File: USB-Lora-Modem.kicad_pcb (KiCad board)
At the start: 4 copper layers, 38.5 x 50.5 mm, 29 parts, among them J2 USB_JUMPER, SW1 KILL_SWITCH, U1 E22-900T30S, U4 USBLC6-2SC6, U6 TPS62A01ADRL, U7 CH343P

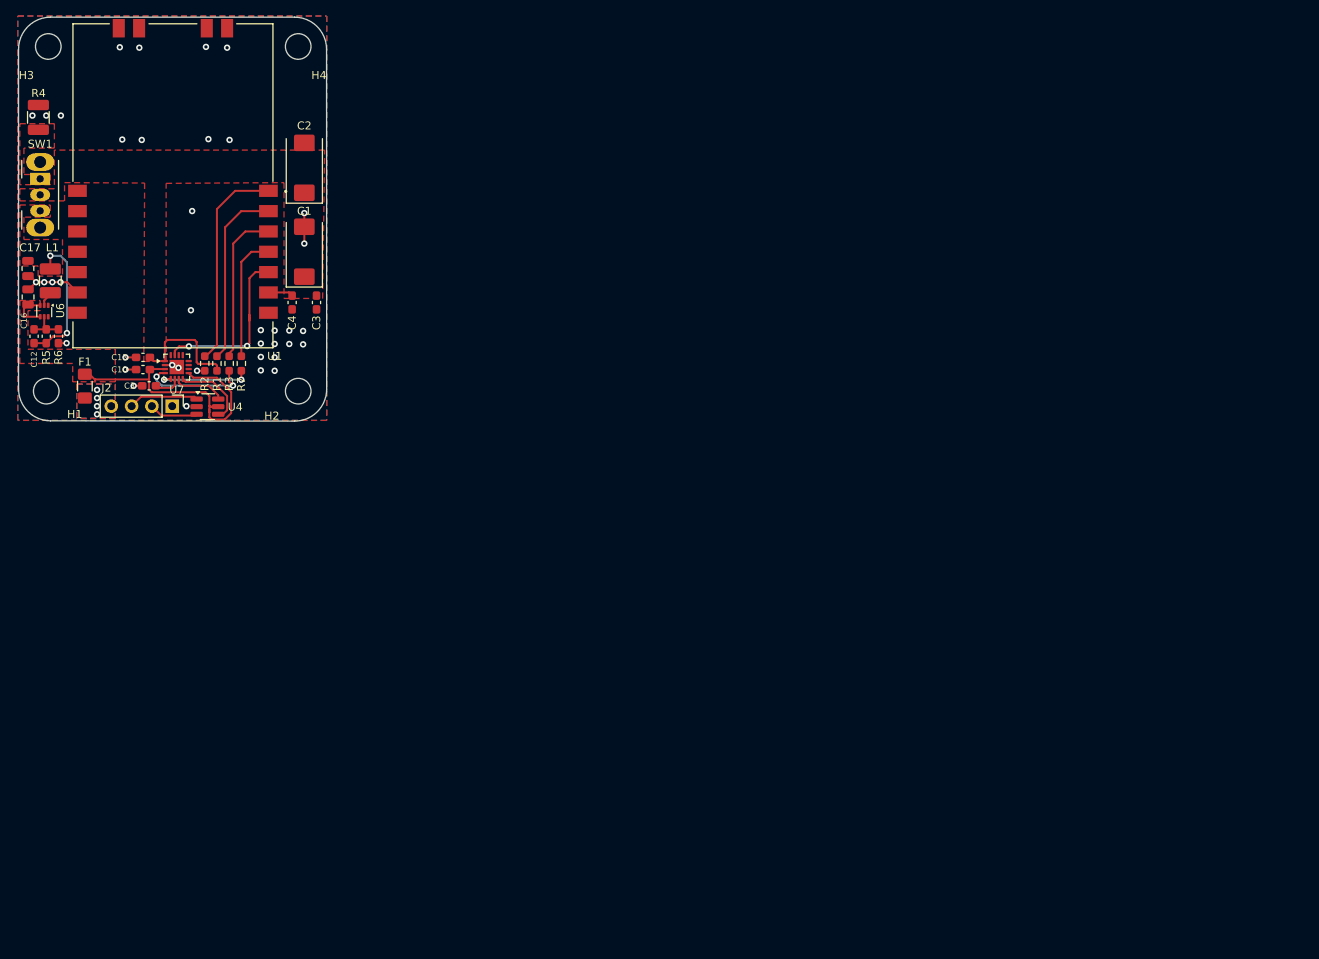
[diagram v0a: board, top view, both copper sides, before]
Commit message: Add files via upload
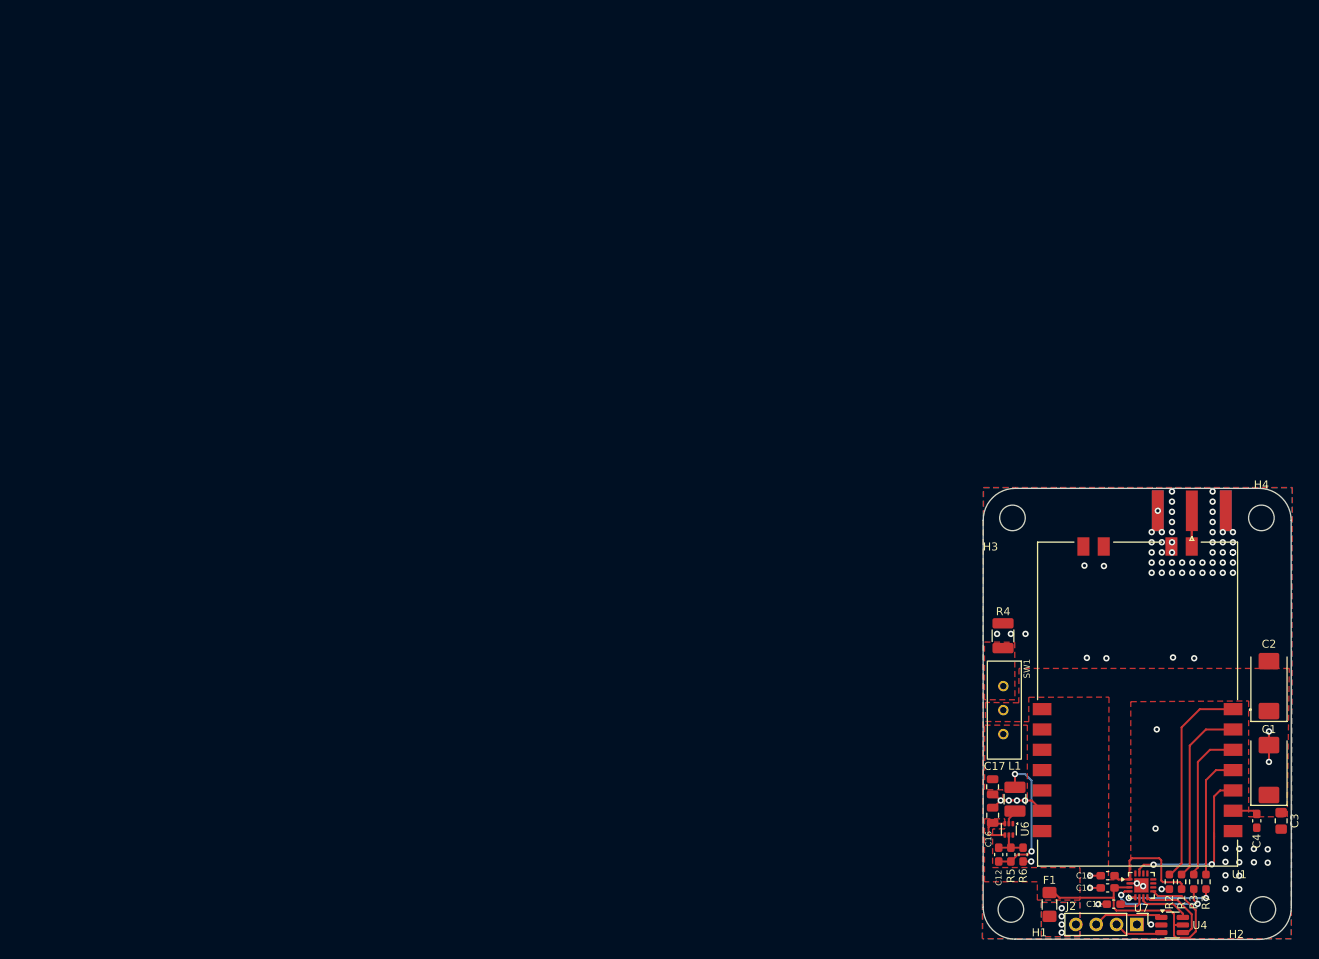
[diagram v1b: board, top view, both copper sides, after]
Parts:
- added J1: Conn_Coaxial, Connector_Coaxial:SMA_Amphenol_132289_EdgeMount, F.Cu at (160.0, 74.8)
- C3: footprint Capacitor_SMD:C_0603_1608Metric_Pad1.08x0.95mm_HandSolder -> Capacitor_SMD:C_0805_2012Metric_Pad1.18x1.45mm_HandSolder
- SW1: footprint Button_Switch_THT:SW_Slide_SPDT_Angled_CK_OS102011MA1Q -> THT_SWITCH:SK-12F04-G050
- moved SW1 137.5 mm to (136.4, 99.7)
- moved C12 136.9 mm to (135.8, 117.8)
- moved C17 136.9 mm to (135.1, 109.3)
- moved H1 136.9 mm to (137.3, 124.6)
- moved R5 136.9 mm to (137.3, 117.8)
- moved R6 136.9 mm to (138.9, 117.8)
- moved C1 136.9 mm to (169.6, 107.2)
- moved C10 136.9 mm to (149.4, 121.9)
- moved C11 136.9 mm to (150.2, 124.0)
- moved C13 136.9 mm to (149.4, 120.4)
- moved C16 136.9 mm to (135.1, 112.9)
- moved C2 136.9 mm to (169.6, 96.7)
- moved C3 136.9 mm to (171.1, 113.6)
- moved C4 136.9 mm to (168.1, 113.6)
- moved F1 136.9 mm to (142.2, 124.0)
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- renumbered C3 to C11
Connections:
- U1 pad 18: unconnected-(U1-ANT-Pad18) -> Net-(J1-In)
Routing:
- net Net-(J1-In): track 0.00 -> 4.47 mm
- net GND: vias 39 -> 83
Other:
- board size 38.5 x 50.5 mm -> 38.5 x 56.4 mm
